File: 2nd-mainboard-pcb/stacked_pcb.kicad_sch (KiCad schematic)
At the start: 17 parts, among them J16 Steckverbinder_Male_Fans, J17 Steckverbinder_Male_Leistung, J18 Steckverbinder_Female_Leistung, J19 Steckverbinder_Male_Motoren, J20 Steckverbinder_Female_Motoren

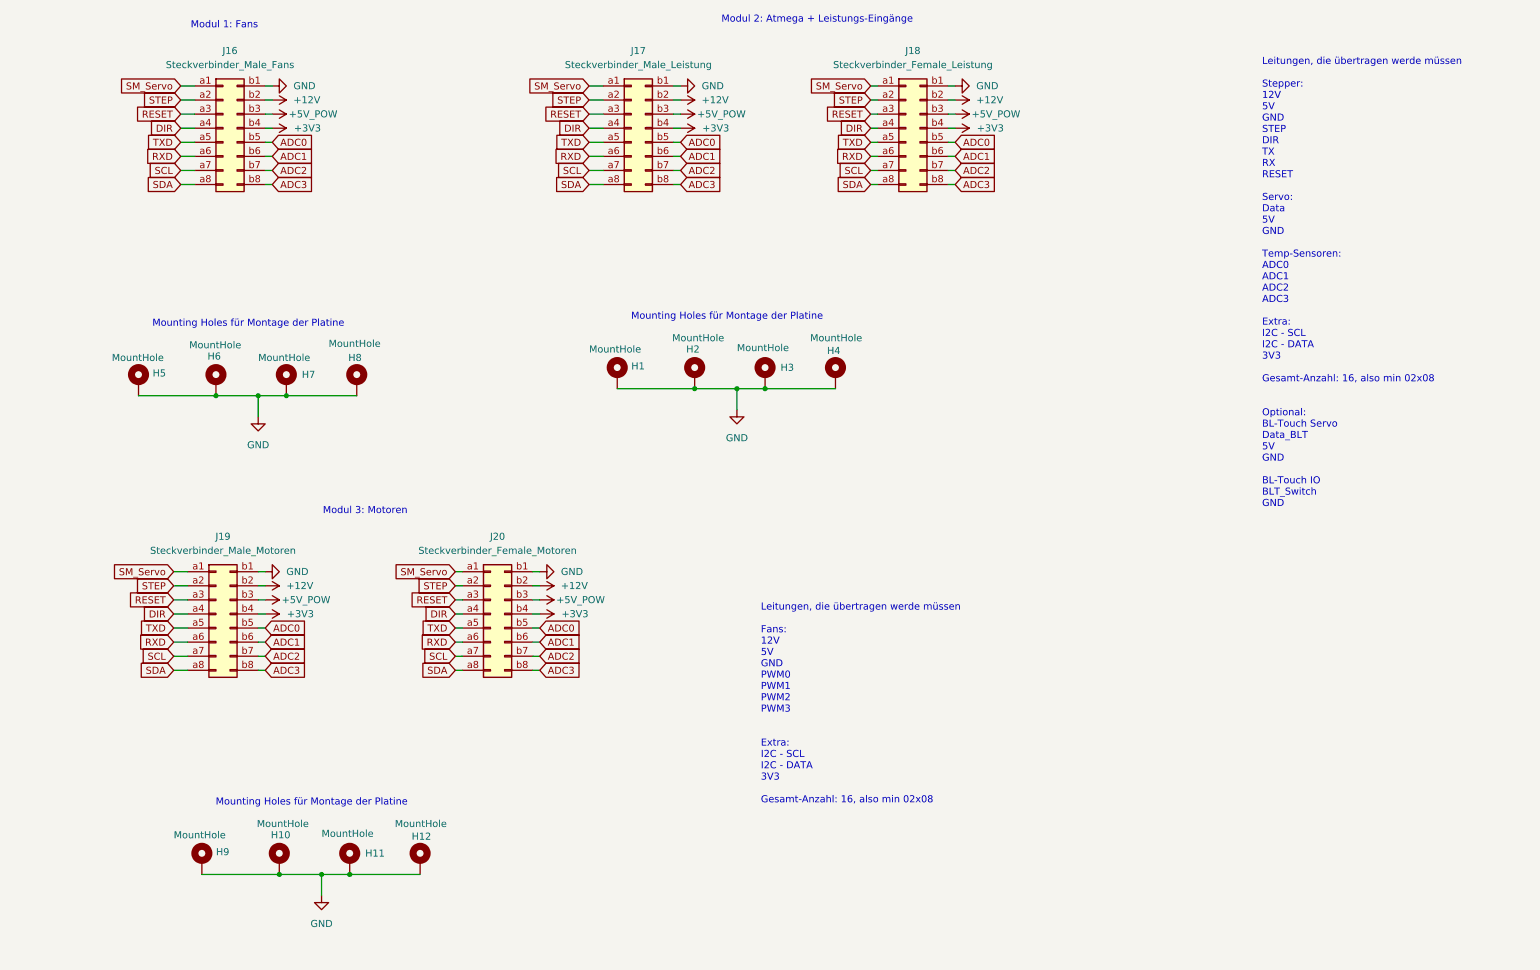
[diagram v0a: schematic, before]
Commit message: new arrangement pcb
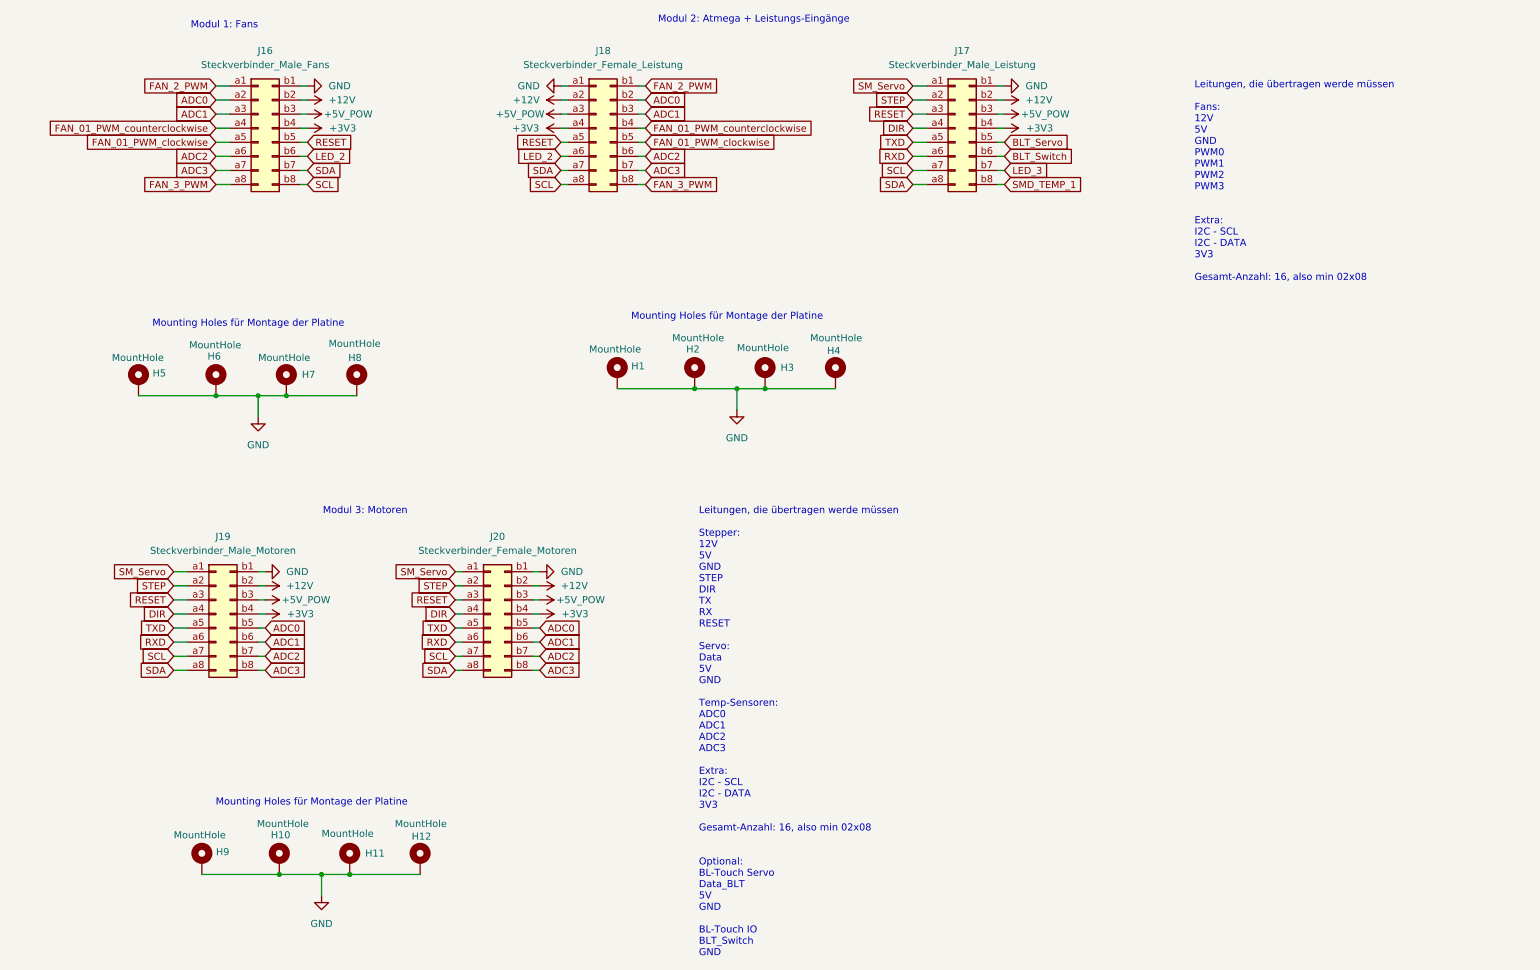
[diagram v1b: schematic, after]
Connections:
- net +12V: now also J18.a2 (Pin_a2); no longer J18.b2 (Pin_b2)
- net +3V3: now also J18.a4 (Pin_a4); no longer J18.b4 (Pin_b4)
- net +5V_POW: now also J18.a3 (Pin_a3); no longer J18.b3 (Pin_b3)
- net ADC0: now also J16.a2 (Pin_a2), J18.b2 (Pin_b2); no longer J16.b5 (Pin_b5), J17.b5 (Pin_b5), J18.b5 (Pin_b5)
- net ADC1: now also J16.a3 (Pin_a3), J18.b3 (Pin_b3); no longer J16.b6 (Pin_b6), J17.b6 (Pin_b6), J18.b6 (Pin_b6)
- net ADC2: now also J16.a6 (Pin_a6), J18.b6 (Pin_b6); no longer J16.b7 (Pin_b7), J17.b7 (Pin_b7), J18.b7 (Pin_b7)
- net ADC3: now also J16.a7 (Pin_a7), J18.b7 (Pin_b7); no longer J16.b8 (Pin_b8), J17.b8 (Pin_b8), J18.b8 (Pin_b8)
- net DIR: no longer J16.a4 (Pin_a4), J18.a4 (Pin_a4)
- net GND: now also J18.a1 (Pin_a1); no longer J18.b1 (Pin_b1)
- net RESET: now also J16.b5 (Pin_b5), J18.a5 (Pin_a5); no longer J16.a3 (Pin_a3), J18.a3 (Pin_a3)
- net RXD: no longer J16.a6 (Pin_a6), J18.a6 (Pin_a6)
- net SCL: now also J16.b8 (Pin_b8), J18.a8 (Pin_a8); no longer J16.a7 (Pin_a7), J18.a7 (Pin_a7)
- net SDA: now also J16.b7 (Pin_b7), J18.a7 (Pin_a7); no longer J16.a8 (Pin_a8), J18.a8 (Pin_a8)
- net SM_Servo: no longer J16.a1 (Pin_a1), J18.a1 (Pin_a1)
- net STEP: no longer J16.a2 (Pin_a2), J18.a2 (Pin_a2)
- net TXD: no longer J16.a5 (Pin_a5), J18.a5 (Pin_a5)
- new net BLT_Servo: J17.b5 (Pin_b5)
- new net BLT_Switch: J17.b6 (Pin_b6)
- new net FAN_01_PWM_clockwise: J16.a5 (Pin_a5), J18.b5 (Pin_b5)
- new net FAN_01_PWM_counterclockwise: J16.a4 (Pin_a4), J18.b4 (Pin_b4)
- new net FAN_2_PWM: J16.a1 (Pin_a1), J18.b1 (Pin_b1)
- new net FAN_3_PWM: J16.a8 (Pin_a8), J18.b8 (Pin_b8)
- new net LED_2: J16.b6 (Pin_b6), J18.a6 (Pin_a6)
- new net LED_3: J17.b7 (Pin_b7)
- new net SMD_TEMP_1: J17.b8 (Pin_b8)
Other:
- moved on the sheet: J16, J17, J18
